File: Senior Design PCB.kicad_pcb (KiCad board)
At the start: 2 copper layers, 203.2 x 76.2 mm, 61 parts, among them J1 Conn_01x02, J10 Conn_01x02, J11 Conn_01x02, J2 Conn_01x02, J3 Raspberry_Pi_Zero_2W, J4 Conn_01x08, J8 Conn_01x02, J9 Conn_01x02, U1 LM2678SX-5.0/NOPB, U2 MCP3008, U3 MAX38890

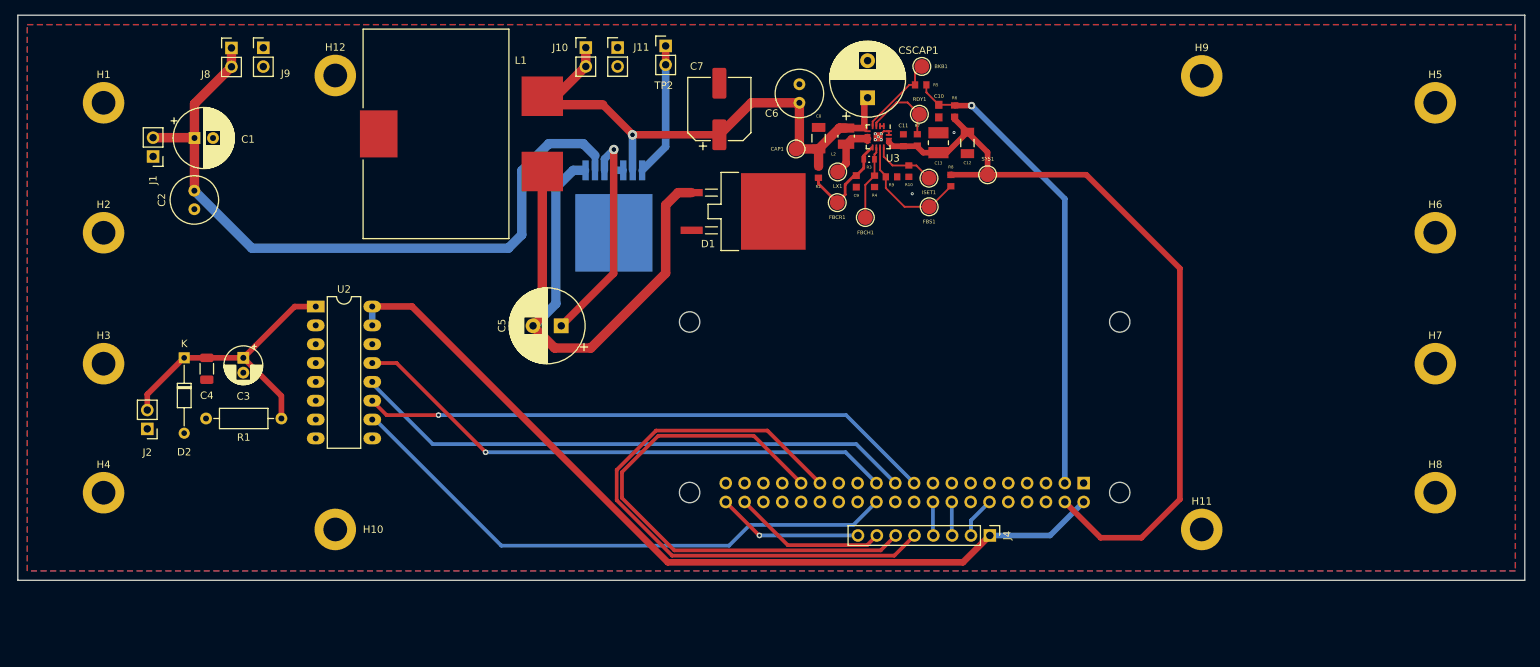
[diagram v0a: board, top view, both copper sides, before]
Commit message: Final files added to 'most recent files' branch.
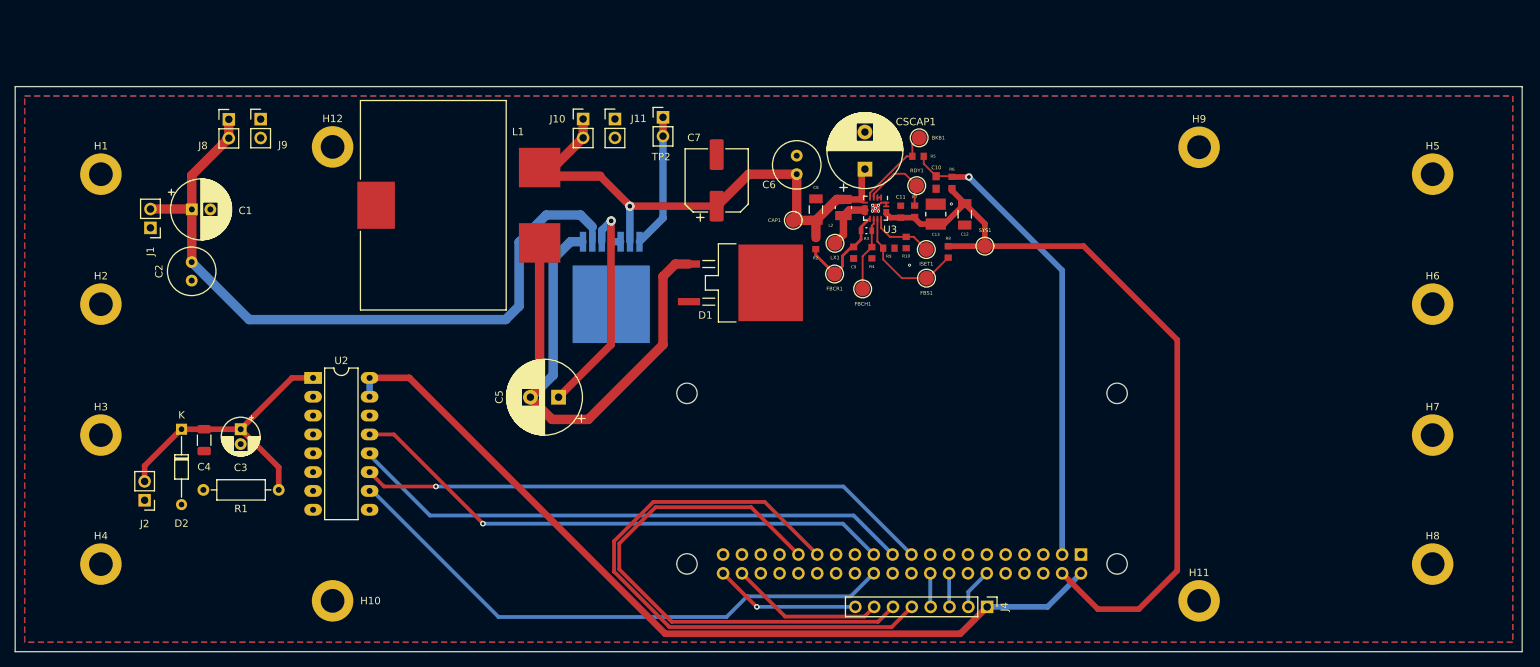
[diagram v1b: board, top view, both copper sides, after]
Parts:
- moved C4 9.63 mm to (70.8, 108.1)
- moved R4 9.63 mm to (160.9, 82.8)
- moved R9 9.63 mm to (163.2, 82.2)
- moved BKB1 9.63 mm to (167.3, 67.3)
- moved C12 9.63 mm to (173.4, 77.6)
- moved C9 9.63 mm to (158.4, 82.8)
- moved FBCR1 9.63 mm to (155.9, 85.7)
- moved H4 9.63 mm to (56.9, 124.8)
- moved H8 9.63 mm to (236.5, 124.8)
- moved J1 9.63 mm to (63.6, 79.5)
- moved R1 9.63 mm to (80.9, 114.8)
- moved R10 9.63 mm to (165.5, 81.5)
- moved R3 9.63 mm to (160.1, 79.9)
- moved RDY1 9.63 mm to (166.9, 73.8)
- moved U1 9.63 mm to (125.7, 89.6)
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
